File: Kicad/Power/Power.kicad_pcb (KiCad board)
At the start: 2 copper layers, 4 parts, among them U1 L7805

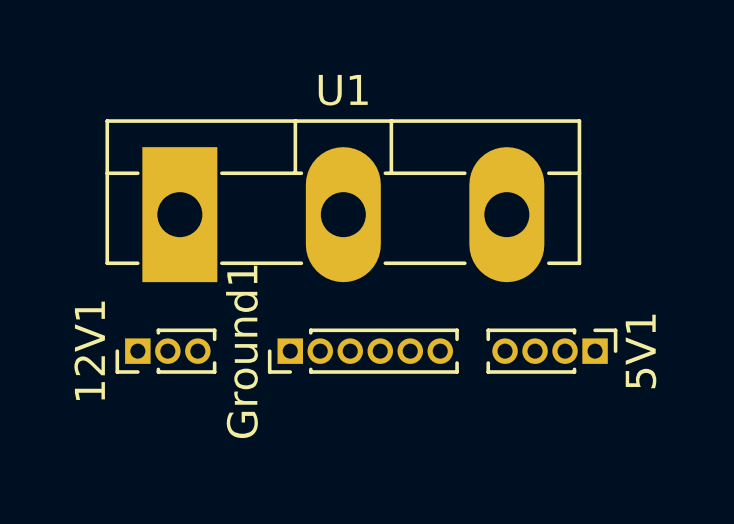
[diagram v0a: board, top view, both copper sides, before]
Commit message: Update
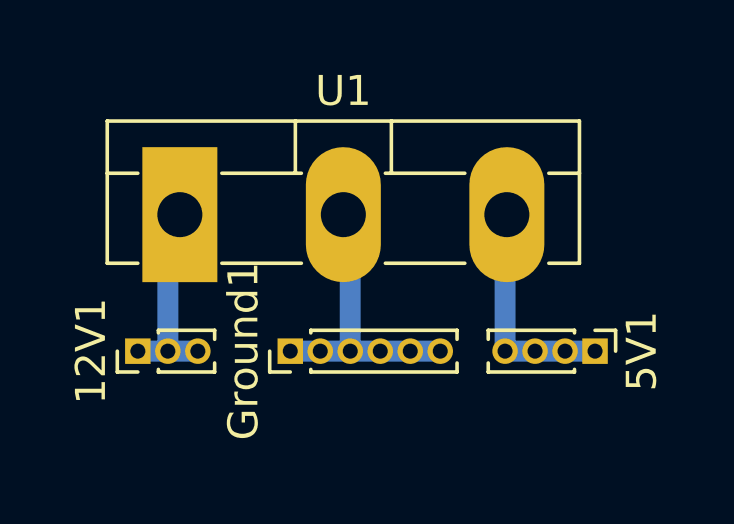
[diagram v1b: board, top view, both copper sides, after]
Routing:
- net Net-(Ground1-Pad1): track 0.00 -> 9.65 mm
- net Net-(U1-Pad3): track 0.00 -> 7.57 mm
- net Net-(12V1-Pad1): track 0.00 -> 6.72 mm
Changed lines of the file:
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@@
   )
   (setup
+    (stackup
+      (layer "F.SilkS" (type "Top Silk Screen"))
+      (layer "F.Paste" (type "Top Solder Paste"))
+      (layer "F.Mask" (type "Top Solder Mask") (thickness 0.01))
+      (layer "F.Cu" (type "copper") (thickness 0.035))
+      (layer "dielectric 1" (type "core") (thickness 1.51) (material "FR4") (epsilon_r 4.5) (loss_tangent 0.02))
+      (layer "B.Cu" (type "copper") (thickness 0.035))
+      (layer "B.Mask" (type "Bottom Solder Mask") (thickness 0.01))
+      (layer "B.Paste" (type "Bottom Solder Paste"))
+      (layer "B.SilkS" (type "Bottom Silk Screen"))
+      (copper_finish "None")
+      (dielectric_constraints no)
+    )
     (pad_to_mask_clearance 0)
     (pcbplotparams
@@
     )
   )
+  (segment (start 131.62 56.47) (end 131.68 56.41) (width 0.7) (layer "B.Cu") (net 1))
+  (segment (start 132.62 60.96) (end 133.62 60.96) (width 0.7) (layer "B.Cu") (net 1))
+  (segment (start 131.62 60.96) (end 131.62 56.47) (width 0.7) (layer "B.Cu") (net 1))
+  (segment (start 133.62 60.96) (end 134.62 60.96) (width 0.7) (layer "B.Cu") (net 1))
+  (segment (start 131.62 60.96) (end 132.62 60.96) (width 0.7) (layer "B.Cu") (net 1))
+  (segment (start 120.38 56.81) (end 120.78 56.41) (width 0.7) (layer "B.Cu") (net 2))
+  (segment (start 119.38 60.96) (end 120.38 60.96) (width 0.7) (layer "B.Cu") (net 2))
+  (segment (start 120.38 60.96) (end 120.38 56.81) (width 0.7) (layer "B.Cu") (net 2))
+  (segment (start 121.38 60.96) (end 120.38 60.96) (width 0.7) (layer "B.Cu") (net 2))
+  (segment (start 126.46 60.96) (end 126.46 56.64) (width 0.7) (layer "B.Cu") (net 3))
+  (segment (start 128.46 60.96) (end 129.46 60.96) (width 0.7) (layer "B.Cu") (net 3))
+  (segment (start 126.46 56.64) (end 126.23 56.41) (width 0.7) (layer "B.Cu") (net 3))
+  (segment (start 126.46 60.96) (end 127.46 60.96) (width 0.7) (layer "B.Cu") (net 3))
+  (segment (start 124.46 60.96) (end 125.46 60.96) (width 0.7) (layer "B.Cu") (net 3))
+  (segment (start 125.46 60.96) (end 126.46 60.96) (width 0.7) (layer "B.Cu") (net 3))
+  (segment (start 127.46 60.96) (end 128.46 60.96) (width 0.7) (layer "B.Cu") (net 3))
 )
